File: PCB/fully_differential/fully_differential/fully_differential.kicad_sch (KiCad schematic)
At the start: 38 parts, among them U1 LM741, U2 LM741, U3 LM741, U4 LM741, U5 LM324, U6 AD8138, U7 LM324

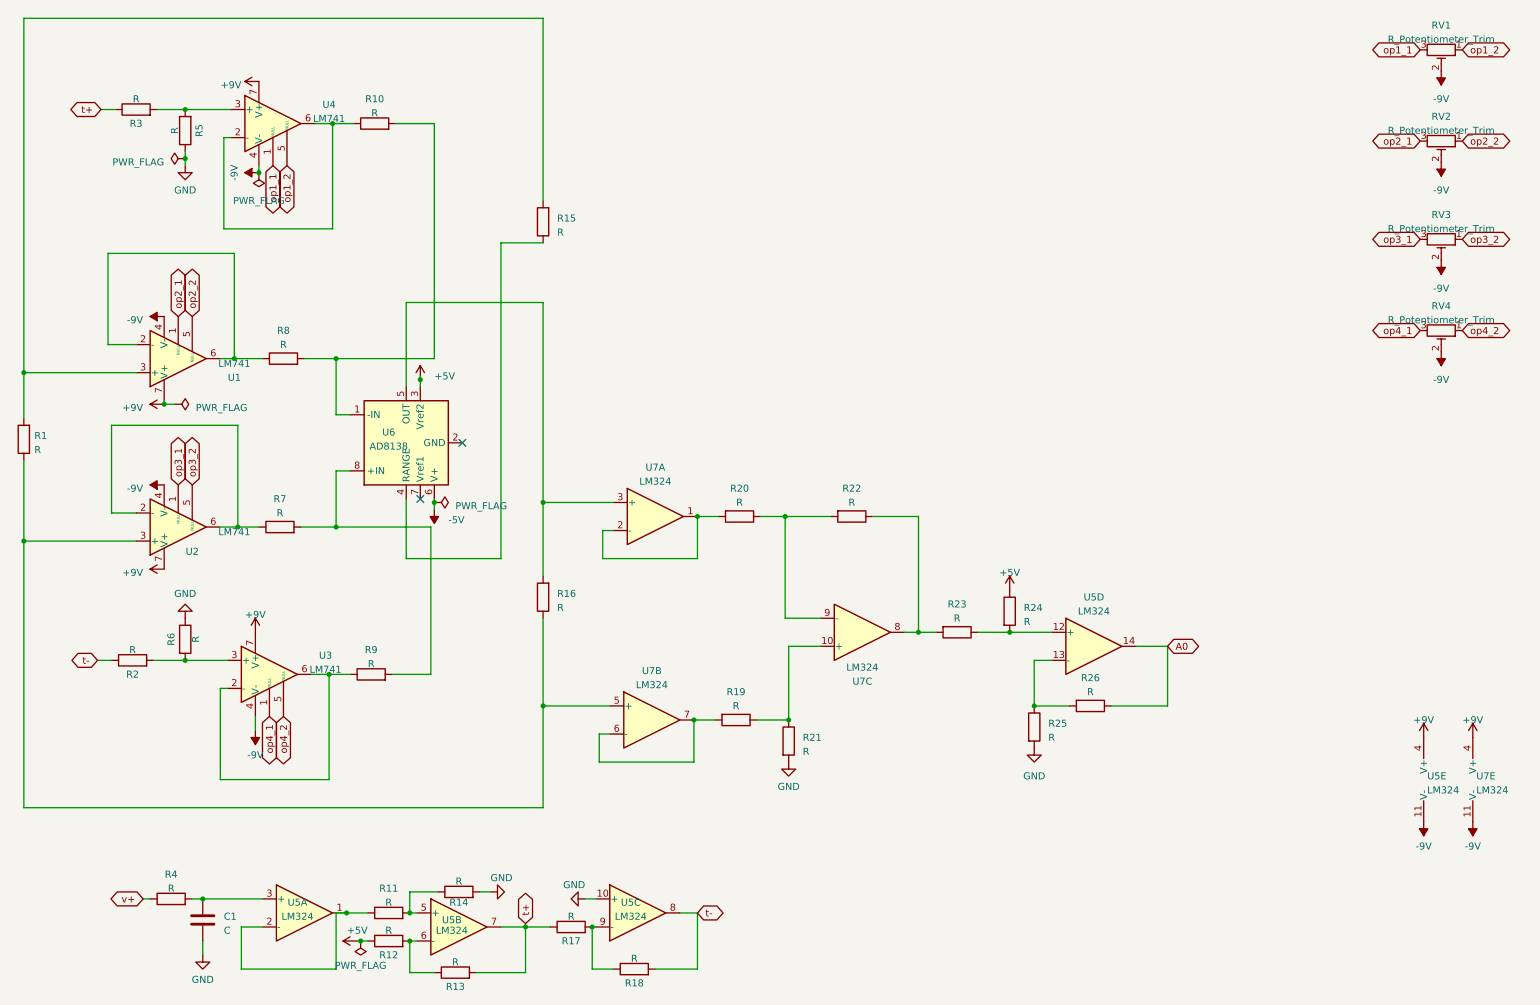
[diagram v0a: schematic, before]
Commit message: new pcb
falta validar para impressao
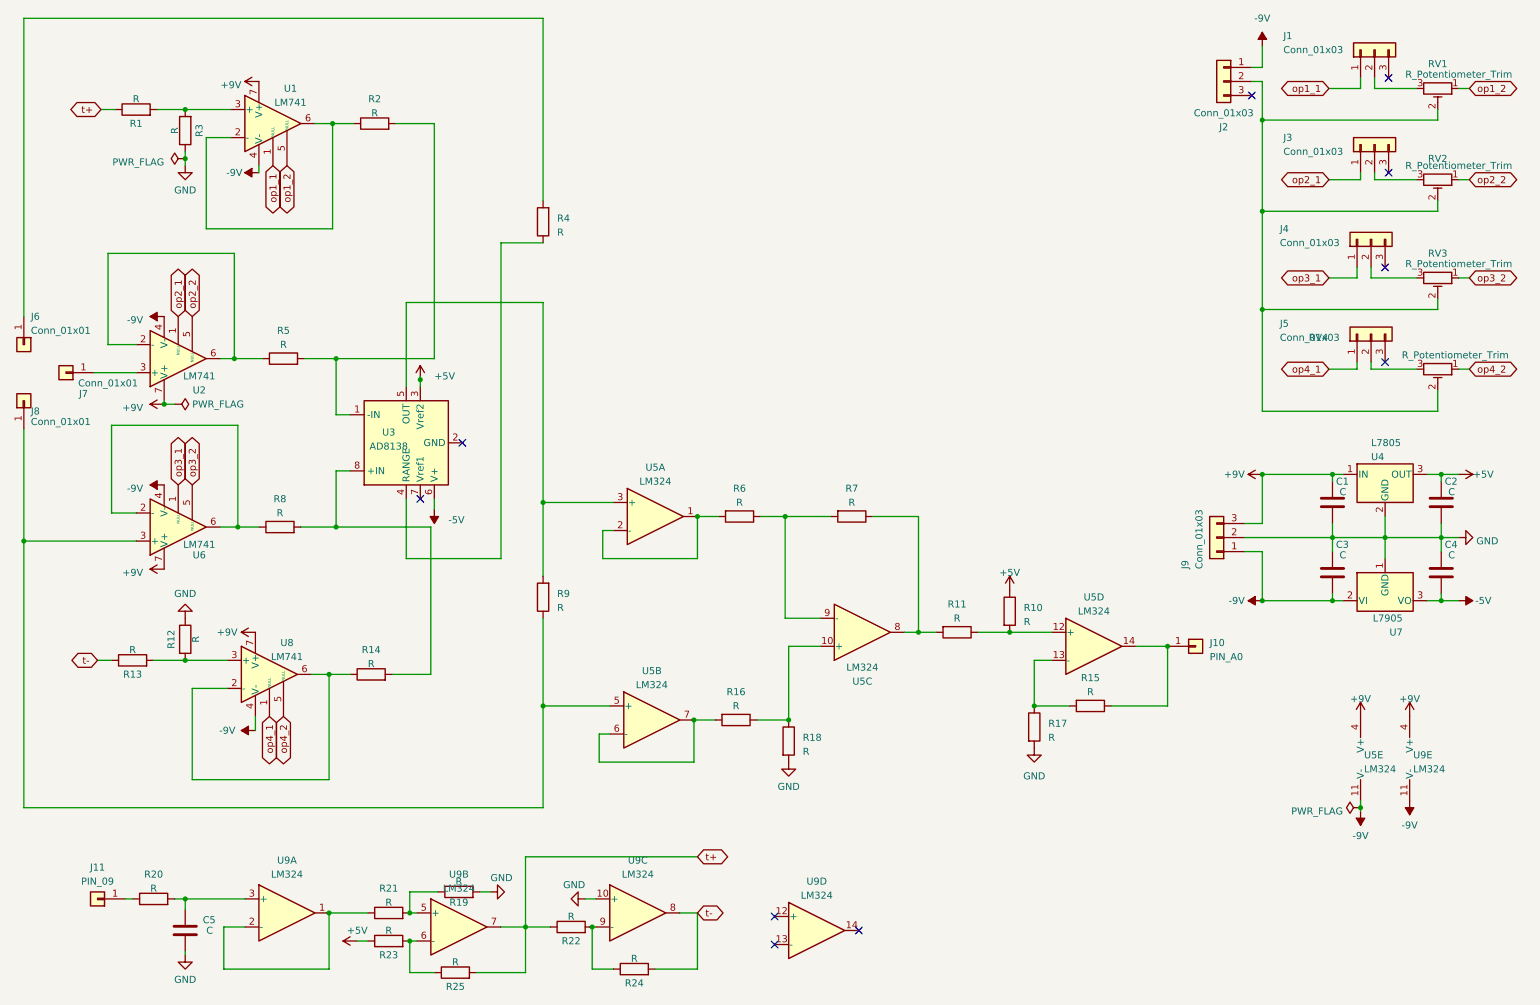
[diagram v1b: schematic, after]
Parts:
- removed R1: R, Resistor_THT:R_Axial_DIN0207_L6.3mm_D2.5mm_P10.16mm_Horizontal, symbol Device:R
- removed unit 1 of U5
- removed unit 2 of U5
- removed unit 3 of U5
- removed unit 5 of U7
- added C1, C2, C3, C4: C, Capacitor_THT:CP_Radial_D5.0mm_P2.00mm, symbol Device:C
- added J1, J2, J3, J4, J5: Conn_01x03, Connector_PinHeader_2.54mm:PinHeader_1x03_P2.54mm_Vertical, symbol Connector_Generic:Conn_01x03
- added J10: PIN_A0, Connector_PinHeader_2.54mm:PinHeader_1x01_P2.54mm_Vertical, symbol Connector_Generic:Conn_01x01
- added J11: PIN_09, Connector_PinHeader_2.54mm:PinHeader_1x01_P2.54mm_Vertical, symbol Connector_Generic:Conn_01x01
- added J6, J7, J8: Conn_01x01, Connector_PinHeader_2.54mm:PinHeader_1x01_P2.54mm_Vertical, symbol Connector_Generic:Conn_01x01
- added J9: Conn_01x03, Connector_Stocko:Stocko_MKS_1653-6-0-303_1x3_P2.50mm_Vertical, symbol Connector_Generic:Conn_01x03
- added U4: L7805, l7805:TO255P1020X450X2000-3, symbol Regulator_Linear:L7805
- added U7: L7905, TO255P1020X450X2000-3, symbol Regulator_Linear:L7905
- added U9: LM324, lm324:DIP825W47P254L1917H533Q14, symbol Amplifier_Operational:LM324
- C5: renamed from C1; footprint Capacitor_THT:C_Rect_L24.0mm_W7.0mm_P22.50mm_MKT -> Capacitor_THT:C_Rect_L19.0mm_W6.0mm_P15.00mm_MKS4
- RV1, RV2, RV3, RV4: footprint Potentiometer_THT:Potentiometer_Runtron_RM-065_Vertical -> Potentiometer_THT:Potentiometer_Bourns_3296W_Vertical
- renumbered R3 to R1, R24 to R10, R23 to R11, R6 to R12, R2 to R13, R9 to R14, R26 to R15, R19 to R16, R25 to R17, R21 to R18, R14 to R19, R10 to R2, R4 to R20, R11 to R21, R17 to R22, R12 to R23, R18 to R24, R13 to R25, R5 to R3, R15 to R4, R8 to R5, R20 to R6, R22 to R7, R7 to R8, R16 to R9, U4 to U1, U1 to U2, U6 to U3, U7 to U5, U2 to U6, U3 to U8
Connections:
- net +5V: now also C2.1, U4.3 (OUT)
- net +9V: now also C1.1, J9.3 (Pin_3), U4.1 (IN), U9.4 (V+)
- net -5V: now also C4.2, U7.3 (VO)
- net -9V: now also C3.2, J2.1 (Pin_1), J9.1 (Pin_1), U7.2 (VI), U9.11 (V-); no longer RV1.2, RV2.2, RV3.2, RV4.2
- net GND: now also C1.2, C2.2, C3.1, C4.1, J9.2 (Pin_2), U4.2 (GND), U7.1 (GND), U9.10 (+)
- net op1_1: now also J1.1 (Pin_1); no longer RV1.3
- net op2_1: now also J3.1 (Pin_1); no longer RV2.3
- net op3_1: now also J4.1 (Pin_1); no longer RV3.3
- net op4_1: now also J5.1 (Pin_1); no longer RV4.3
- net t+: now also U9.7
- net t-: now also U9.8
- net at R4.2: now also J6.1 (Pin_1); no longer U2.3 (+)
- net at R9.1, U5.5 (+), U6.3 (+): now also J8.1 (Pin_1)
- net at R22.2, R24.1: now also U9.9 (-)
- net at R23.2, R25.1: now also U9.6 (-)
- net at R19.1, R21.2: now also U9.5 (+)
- net at R21.1: now also U9.1, U9.2 (-)
- net at C5.1, R20.2: now also U9.3 (+)
- net A0: no longer names the net of R15.1, U5.14
- net A0: now also J10.1 (Pin_1)
- net v+: no longer names the net of R20.1
- net v+: now also J11.1 (Pin_1)
- new net: J4.2 (Pin_2), RV3.3
- new net: J1.2 (Pin_2), RV1.3
- new net: J5.2 (Pin_2), RV4.3
- new net: J2.2 (Pin_2), RV1.2, RV2.2, RV3.2, RV4.2
- new net: J7.1 (Pin_1), U2.3 (+)
- new net: J3.2 (Pin_2), RV2.3
- no-connect marks 2 -> 10
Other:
- company: (none) -> Felipe Avila Silva
- title: (none) -> Fully Differential Potentiostat
- moved on the sheet: C5, R20, RV1, RV2, RV3, RV4, U5E
